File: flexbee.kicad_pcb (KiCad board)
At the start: 4 copper layers, 30.7 x 17.6 mm, 68 parts, among them J1 Conn_01x12_Male, J2 Conn_01x12_Male, U1 SSD210, U2 ea3056, U3 spinor, Y1 Crystal_GND24

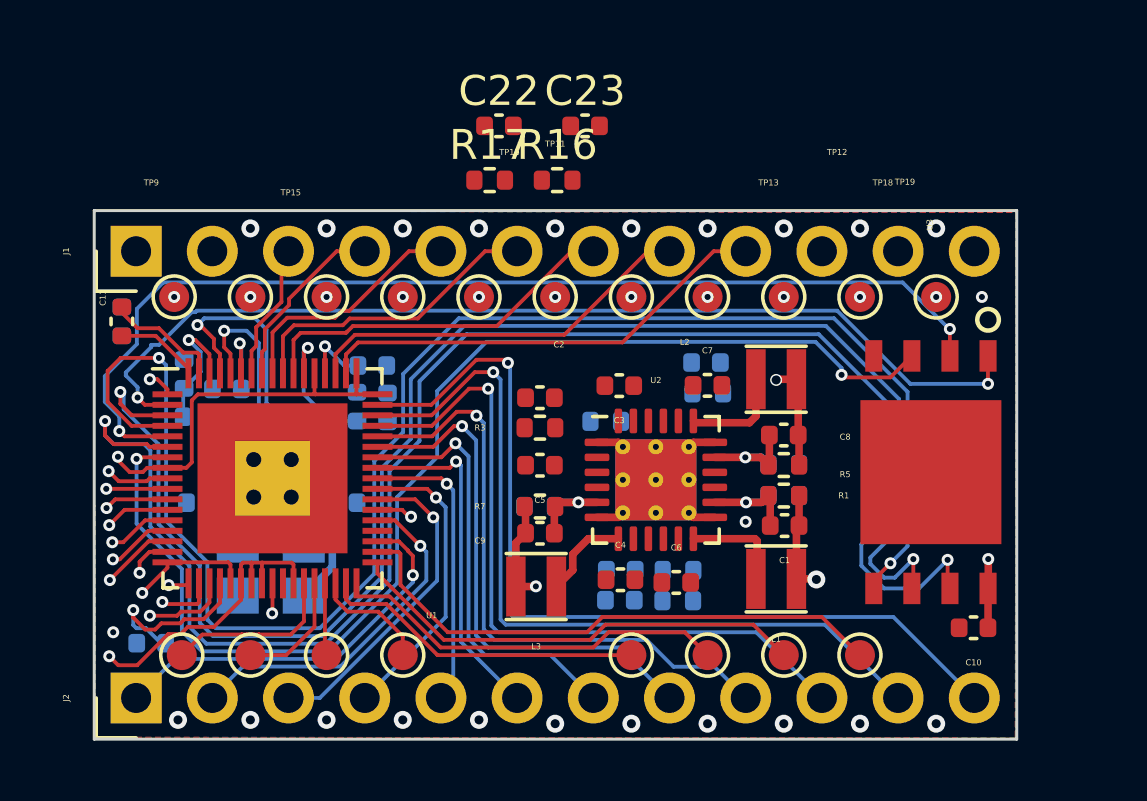
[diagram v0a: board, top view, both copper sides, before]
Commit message: Add files via upload
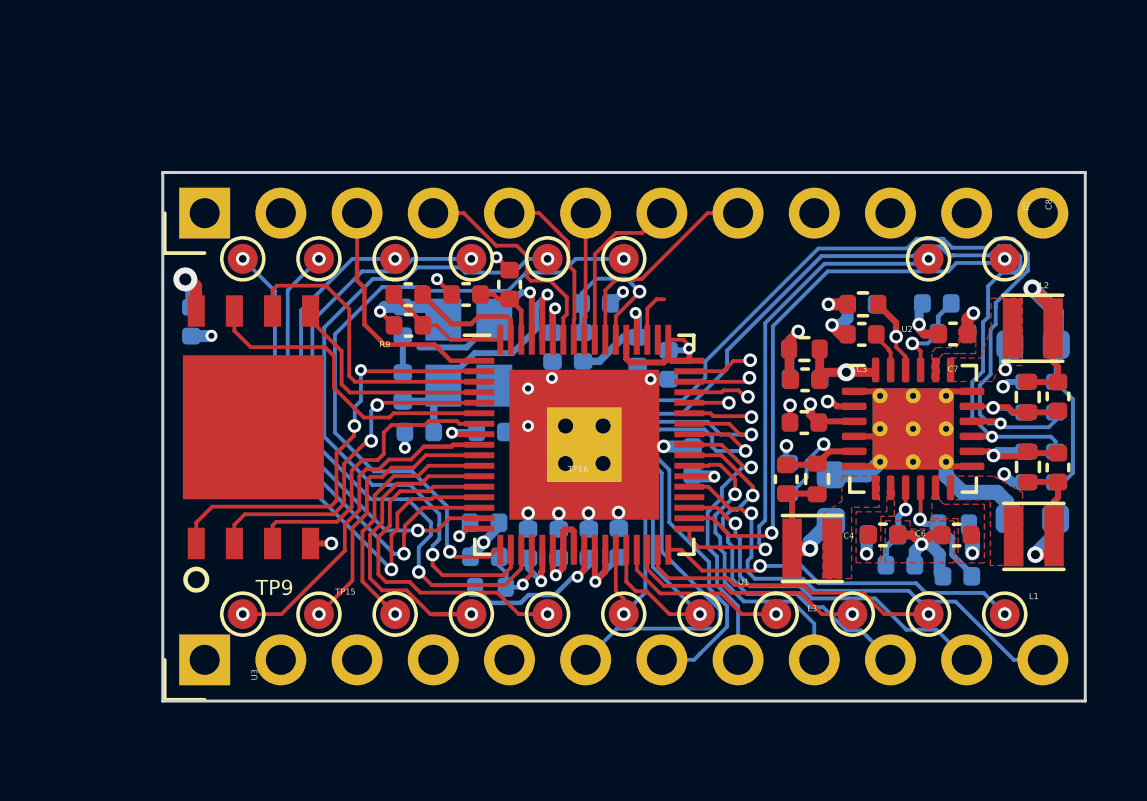
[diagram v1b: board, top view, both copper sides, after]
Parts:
- added C24: C, Capacitor_SMD:C_0402_1005Metric, B.Cu at (142.6, 96.1)
- added C25: C, Capacitor_SMD:C_0402_1005Metric, B.Cu at (143.6, 96.1)
- added C26: C, Capacitor_SMD:C_0402_1005Metric, B.Cu at (140.1, 95.4)
- added C27: C, Capacitor_SMD:C_0402_1005Metric, B.Cu at (146.3, 90.1)
- added C28: C, Capacitor_SMD:C_0402_1005Metric, B.Cu at (140.4, 92.4)
- added C29: C, Capacitor_SMD:C_0402_1005Metric, B.Cu at (142.4, 89.6)
- added C30: C, Capacitor_SMD:C_0402_1005Metric, B.Cu at (147.1, 93.3)
- added C31: C, Capacitor_SMD:C_0603_1608Metric, B.Cu at (158.4, 95.3)
- added C32: C, Capacitor_SMD:C_0603_1608Metric, B.Cu at (151.7, 94.6)
- added C33: C, Capacitor_SMD:C_0603_1608Metric, B.Cu at (158.4, 89.5)
- added R18: R, Resistor_SMD:R_0402_1005Metric, B.Cu at (159.2, 93.5)
- added R19: R, Resistor_SMD:R_0402_1005Metric, B.Cu at (159.2, 91.2)
- C10, C22, C23, R16: moved to B.Cu
- C13, R11, R9: moved to F.Cu
- moved C10 28.0 mm to (130.4, 88.7), turned to -90 degrees
- moved U3 22.6 mm to (132.4, 92.2), turned to 90 degrees
- moved TP1 17.3 mm to (147.3, 98.5)
- moved TP14 15.5 mm to (139.7, 86.6)
- moved TP2 15.0 mm to (149.9, 98.5)
- moved TP6 15.0 mm to (152.4, 98.5)
- moved C22 14.5 mm to (144.6, 96.1), turned to 90 degrees
- moved TP4 14.1 mm to (154.9, 86.6)
- moved TP8 14.1 mm to (157.5, 86.6)
- moved R16 13.8 mm to (140.3, 97.6)
- moved R17 13.1 mm to (152.8, 88.1)
- moved TP5 12.5 mm to (144.8, 98.5)
- moved C16 11.5 mm to (140.2, 96.5)
- moved C14 11.3 mm to (141.6, 96.1), turned to 90 degrees
- moved C13 11.3 mm to (141.0, 87.5)
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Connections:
- J1 pad 1: VCC -> +3V3
- J1 pad 10: /lineout -> /usb_dp
- J1 pad 11: +3V3 -> VCC
- J1 pad 3: /sar_gpio0 -> /lineout
- J1 pad 4: /sar_gpio1 -> /sar_gpio0
- J1 pad 5: /sar_gpio2 -> /sar_gpio1
- J1 pad 6: /uart_rx -> /sar_gpio2
- J1 pad 7: /uart_tx -> /uart_rx
- J1 pad 8: /usb_dm -> /uart_tx
- J1 pad 9: /usb_dp -> /usb_dm
- J2 pad 1: /ttl8 -> /ttl21
- J2 pad 10: /ttl19 -> /ttl13
- J2 pad 11: /ttl20 -> /ttl8
- J2 pad 12: /ttl21 -> /ttl11
- J2 pad 2: /ttl11 -> /ttl20
- J2 pad 3: /ttl12 -> /ttl19
- J2 pad 4: /ttl13 -> /ttl18
- J2 pad 5: /ttl14 -> /ttl17
- J2 pad 6: /ttl15 -> /ttl16
- J2 pad 7: /ttl16 -> /ttl15
- J2 pad 8: /ttl17 -> /ttl14
- J2 pad 9: /ttl18 -> /ttl12
- TP1 pad 1: Net-(TP1-Pad1) -> /i2c0_sda
- TP5 pad 1: Net-(TP5-Pad1) -> /i2c0_scl
- U1 pad 29: Net-(TP1-Pad1) -> /i2c0_scl
- U1 pad 30: Net-(TP5-Pad1) -> /i2c0_sda
- U2 pad 15: unconnected-(U2-Pad15) -> /i2c0_sda
- U2 pad 16: unconnected-(U2-Pad16) -> /i2c0_scl
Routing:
- net /flash_mosi: track 53.7 -> 7.93 mm, vias 2 -> 0
- net /flash_hld: track 53.7 -> 10.7 mm, vias 2 -> 0
- net +3V3: track 67.5 -> 25.7 mm, vias 6 -> 8
- net /flash_clk: track 51.7 -> 10.3 mm, vias 2 -> 0
- net /i2c0_sda: track 0.00 -> 37.6 mm, vias 0 -> 2
- net /i2c0_scl: track 0.00 -> 36.9 mm, vias 0 -> 2
- net GND: track 3.70 -> 36.6 mm
- net /flash_wpz: track 40.2 -> 10.1 mm, vias 2 -> 0
- net +1V0: track 48.0 -> 18.6 mm, vias 3 -> 4
- net /flash_miso: track 35.4 -> 11.8 mm
- net /flash_cs: track 33.7 -> 14.5 mm
- net /lineout: track 26.9 -> 8.14 mm, vias 1 -> 0
- net +1V8: track 29.2 -> 13.2 mm, vias 2 -> 3
- net /usb_dp: track 15.4 -> 0.00 mm
- net Net-(TP14-Pad1): track 34.7 -> 21.5 mm
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- added copper zone on In2.Cu, net +1V0
- added copper zone on In2.Cu, net +1V8
- added copper zone on In2.Cu, net +3V3
- added copper zone on F.Cu, net Net-(L1-Pad2)
- added copper zone on F.Cu, net Net-(L2-Pad1)
- added copper zone on F.Cu, net Net-(L3-Pad1)
- added copper zone on In2.Cu, net VBUS
- added copper zone on F.Cu, net VCC
- added copper zone on In2.Cu, net VCC
- removed copper zone on B.Cu, net GND
- removed copper zone on In2.Cu, net GND
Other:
- board size 30.7 x 17.6 mm -> 30.8 x 17.6 mm
